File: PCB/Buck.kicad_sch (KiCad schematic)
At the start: 29 parts, among them U12 PTPS548A28RWWR, U13 TLV62569DBV

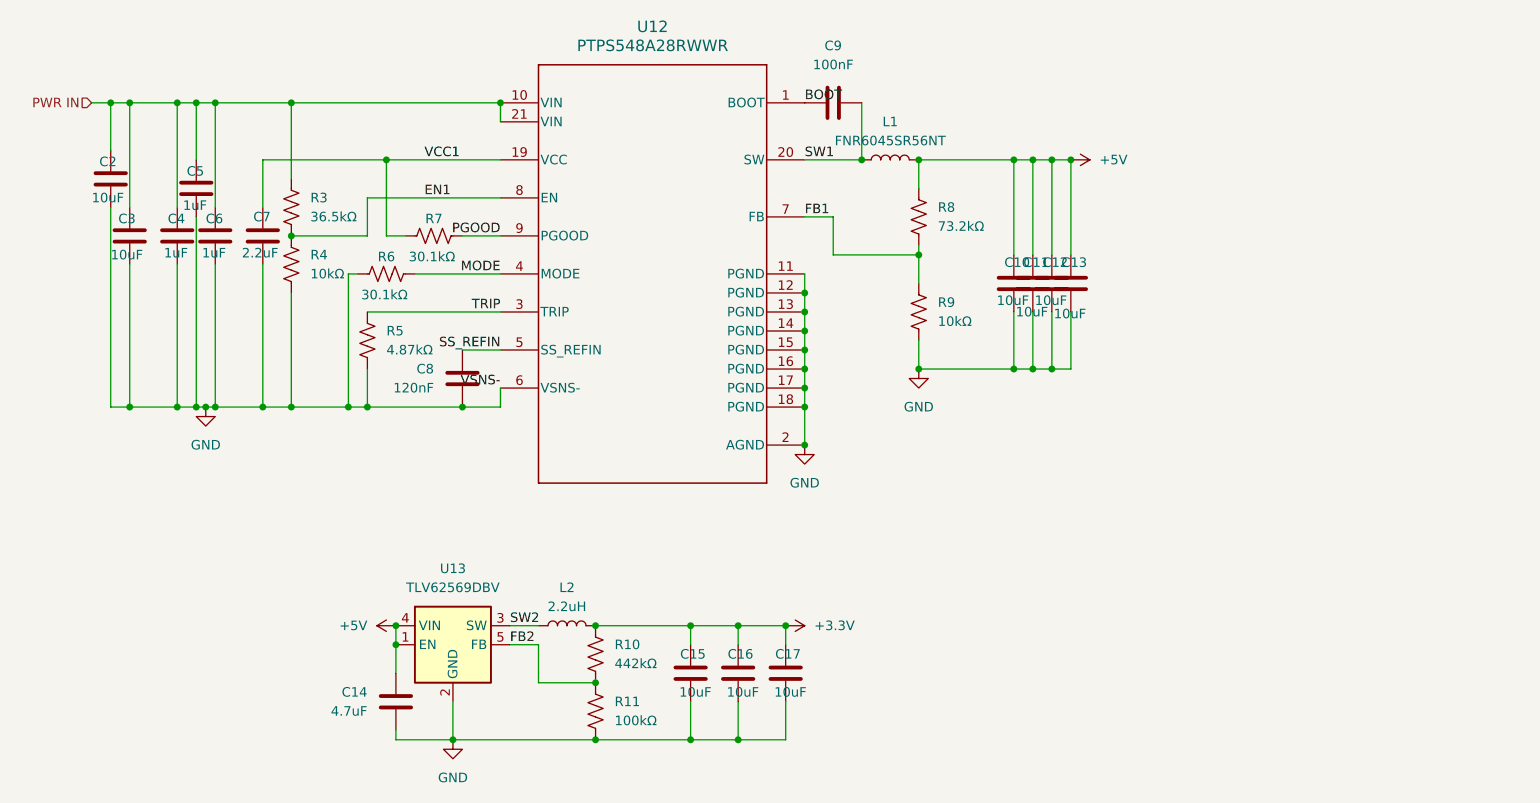
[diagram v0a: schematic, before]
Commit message: Updated PCB
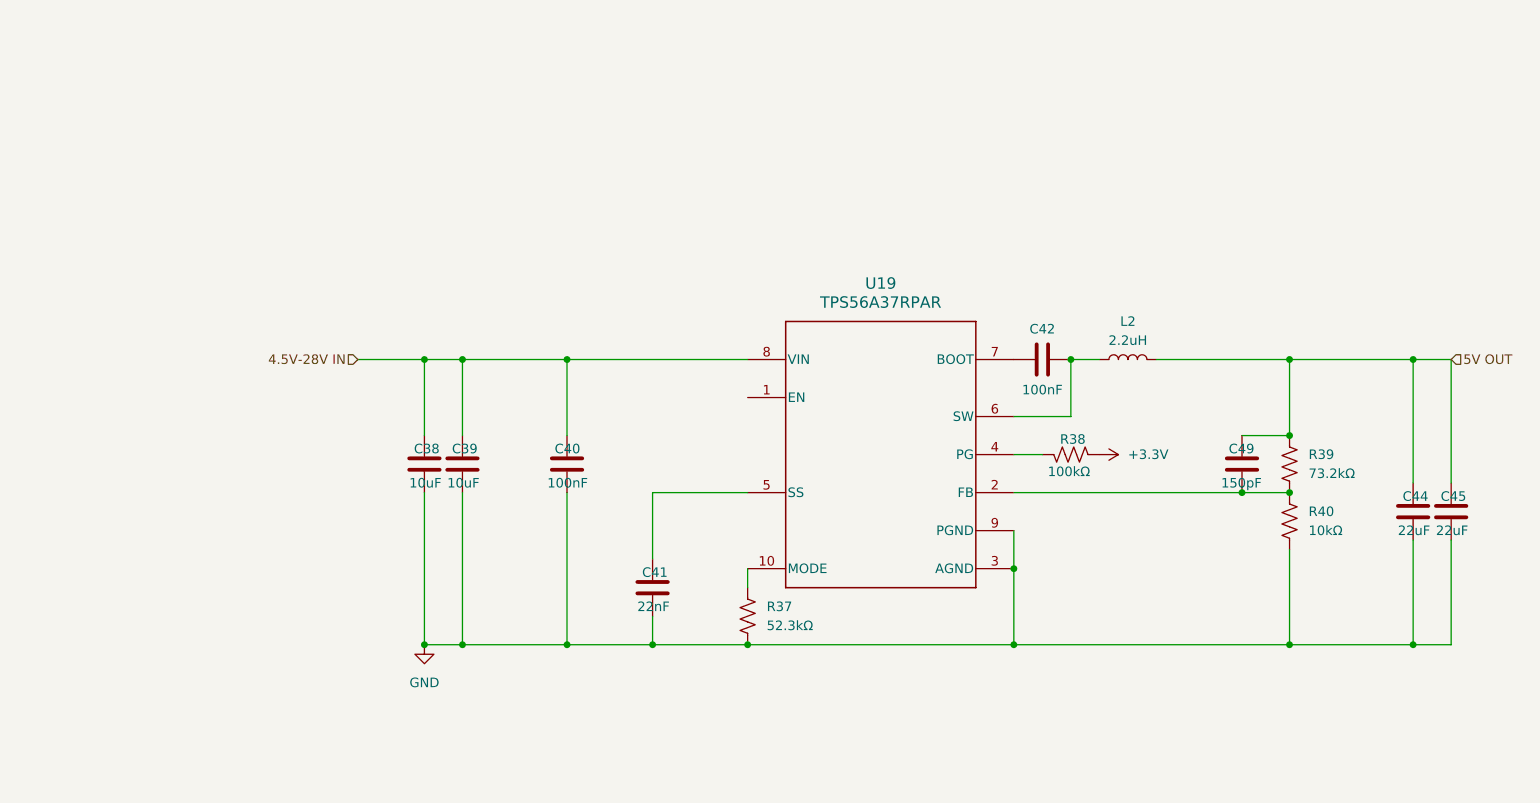
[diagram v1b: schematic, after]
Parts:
- removed C10, C11, C12, C13, C15, C16, C17, C2, C3: 10uF, Capacitor_SMD:C_0402_1005Metric, symbol Device:C
- removed C14: 4.7uF, Capacitor_SMD:C_0402_1005Metric, symbol Device:C
- removed C4, C5, C6: 1uF, Capacitor_SMD:C_0402_1005Metric_Pad0.74x0.62mm_HandSolder, symbol Device:C
- removed C7: 2.2uF, Capacitor_SMD:C_0402_1005Metric, symbol Device:C
- removed C8: 120nF, Capacitor_SMD:C_0402_1005Metric, symbol Device:C
- removed C9: 100nF, Capacitor_SMD:C_0402_1005Metric, symbol Device:C
- removed L1: FNR6045SR56NT, Inductor_SMD:L_Changjiang_FNR6045S, symbol Device:L
- removed R10: 442kΩ, Resistor_SMD:R_0402_1005Metric, symbol Device:R_US
- removed R11: 100kΩ, Resistor_SMD:R_0402_1005Metric, symbol Device:R_US
- removed R3: 36.5kΩ, Resistor_SMD:R_0402_1005Metric, symbol Device:R_US
- removed R4, R9: 10kΩ, Resistor_SMD:R_0402_1005Metric, symbol Device:R_US
- removed R5: 4.87kΩ, Resistor_SMD:R_0402_1005Metric, symbol Device:R_US
- removed R6, R7: 30.1kΩ, Resistor_SMD:R_0402_1005Metric, symbol Device:R_US
- removed R8: 73.2kΩ, Resistor_SMD:R_0402_1005Metric, symbol Device:R_US
- removed U12: PTPS548A28RWWR, Library:RWW0021A, symbol BMS:PTPS548A28RWWR
- removed U13: TLV62569DBV, Package_TO_SOT_SMD:SOT-23-5, symbol Regulator_Switching:TLV62569DBV
- added C38, C39: 10uF, Capacitor_SMD:C_0805_2012Metric_Pad1.18x1.45mm_HandSolder, symbol Device:C
- added C40, C42: 100nF, Capacitor_SMD:C_0603_1608Metric_Pad1.08x0.95mm_HandSolder, symbol Device:C
- added C41: 22nF, Capacitor_SMD:C_0603_1608Metric_Pad1.08x0.95mm_HandSolder, symbol Device:C
- added C44, C45: 22uF, Capacitor_SMD:C_0805_2012Metric_Pad1.18x1.45mm_HandSolder, symbol Device:C
- added C49: 150pF, Capacitor_SMD:C_0603_1608Metric_Pad1.08x0.95mm_HandSolder, symbol Device:C
- added R37: 52.3kΩ, Resistor_SMD:R_0603_1608Metric_Pad0.98x0.95mm_HandSolder, symbol Device:R_US
- added R38: 100kΩ, Resistor_SMD:R_0603_1608Metric_Pad0.98x0.95mm_HandSolder, symbol Device:R_US
- added R39: 73.2kΩ, Resistor_SMD:R_0603_1608Metric_Pad0.98x0.95mm_HandSolder, symbol Device:R_US
- added R40: 10kΩ, Resistor_SMD:R_0603_1608Metric_Pad0.98x0.95mm_HandSolder, symbol Device:R_US
- added U19: TPS56A37RPAR, CM5IO:RPA0010A-MFG, symbol CM5IO:TPS56A37RPAR
- L2: footprint Inductor_SMD:L_Sunlord_SWPA6045S -> Inductor_SMD:L_Coilcraft_XAL7030-222
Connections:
- net +3.3V: now also R38.1; no longer L2.2
- net GND: now also C38.1, C39.1, C40.1, C41.1, C44.1, C45.1, R37.2, R40.2, U19.3 (AGND), U19.9 (PGND)
- net SW2: no longer names the net of L2.1
- net SW2: now also C42.2, U19.6 (SW)
- new net: C42.1, U19.7 (BOOT)
- new net: R37.1, U19.10 (MODE)
- new net: C49.1, R39.2, R40.1, U19.2 (FB)
- new net: R38.2, U19.4 (PG)
- new net: C41.2, U19.5 (SS)
- new net 4.5V-28V IN: C38.2, C39.2, C40.2, U19.8 (VIN)
- new net 5V OUT: C44.2, C45.2, C49.2, L2.2, R39.1
